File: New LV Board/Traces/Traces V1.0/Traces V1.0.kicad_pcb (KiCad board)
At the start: 6 copper layers, 105.7 x 51.8 mm, 15 parts, among them J1 B15B-PH-K-S, J2 B15B-PH-K-S, J3 B15B-PH-K-S, J4 Conn_01x12, J6 Conn_01x12, J7 Conn_01x12

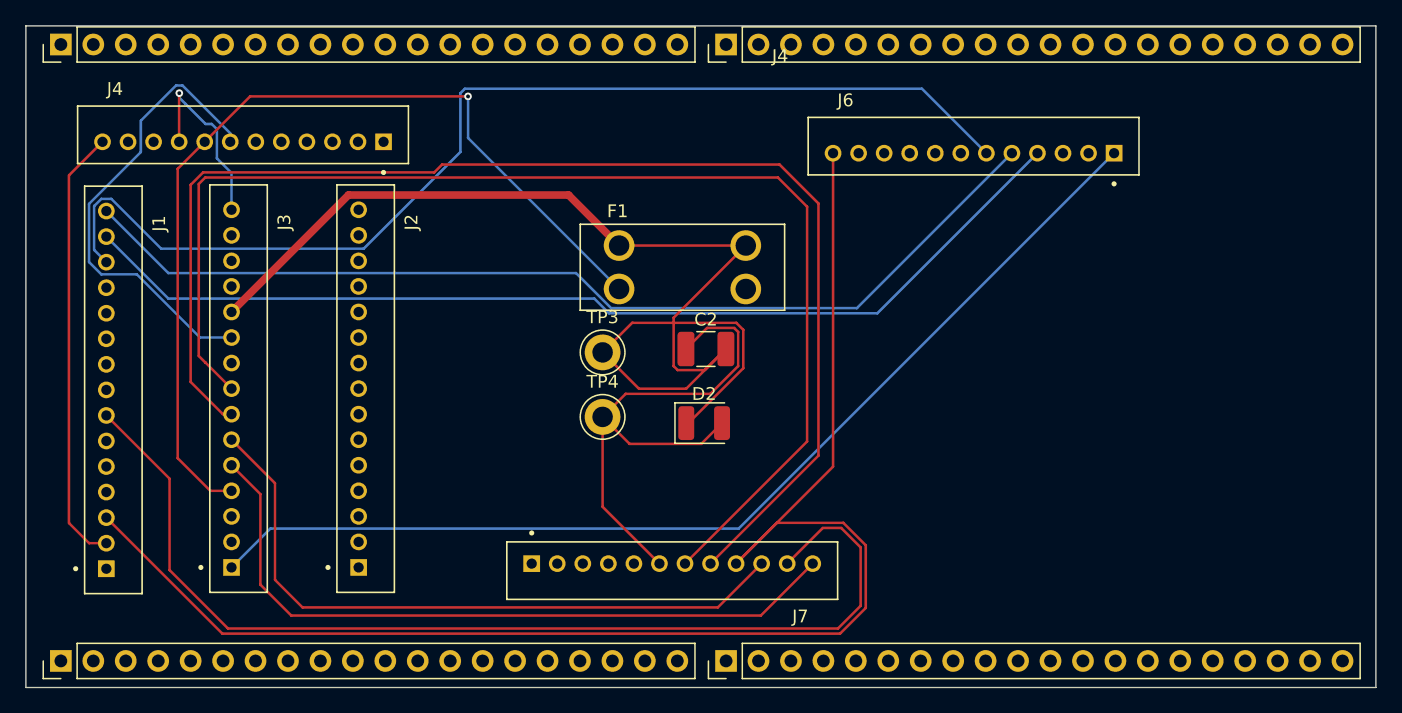
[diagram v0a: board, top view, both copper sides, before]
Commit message: traces probably
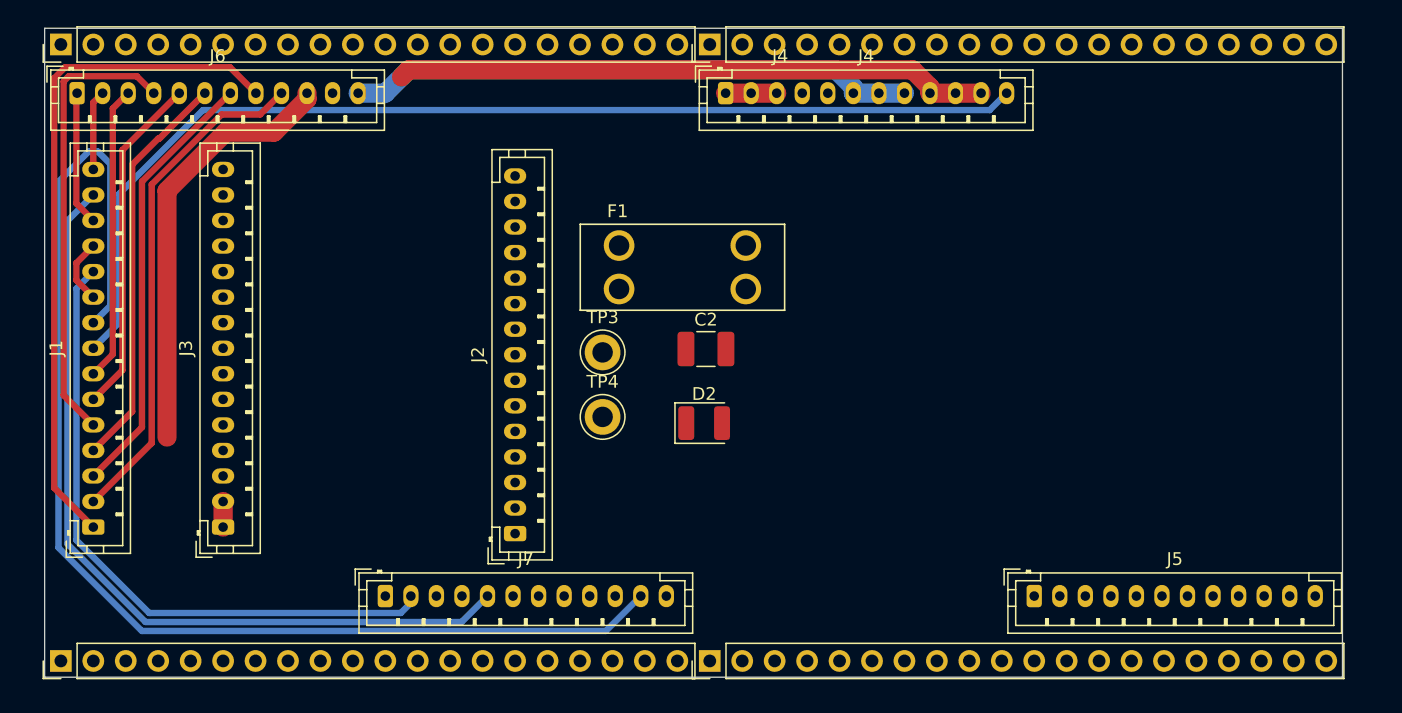
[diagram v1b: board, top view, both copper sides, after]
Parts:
- added J5: B12B-PH-K-S, Connector_JST:JST_PH_B12B-PH-K_1x12_P2.00mm_Vertical, F.Cu at (116.8, 104.1)
- J1, J2, J3: footprint motorsports:JST_B15B-PH-K-S -> Connector_JST:JST_PH_B15B-PH-K_1x15_P2.00mm_Vertical
- J4, J6, J7: value Conn_01x12 -> B12B-PH-K-S; footprint motorsports:JST_B12B-PH-K-S -> Connector_JST:JST_PH_B12B-PH-K_1x12_P2.00mm_Vertical
- moved J6 70.3 mm to (41.9, 64.8)
- moved J4 37.9 mm to (92.7, 64.8)
- moved J7 22.5 mm to (66.0, 104.1), turned to 0 degrees
- moved J2 16.3 mm to (76.2, 99.2), turned to 90 degrees
- moved J3 10.9 mm to (53.3, 98.7), turned to 90 degrees
- moved J1 10.9 mm to (43.2, 98.7), turned to 90 degrees
- moved REF** 1.28 mm to (91.4, 61.0)
- moved REF** 1.28 mm to (91.4, 109.2)
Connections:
- F1 pad 3: Net-(J4-Pin_8) -> Net-(J4-Pin_5)
- F1 pad 4: Net-(J4-Pin_8) -> Net-(J4-Pin_5)
- J1 pad 1: Net-(J6-Pin_11) -> Net-(J6-Pin_8)
- J1 pad 10: Net-(J6-Pin_8) -> Net-(J1-Pad10)
- J1 pad 11: Net-(J6-Pin_9) -> Net-(J7-Pin_2)
- J1 pad 12: Net-(J6-Pin_7) -> Net-(J1-Pad10)
- J1 pad 13: Net-(J6-Pin_6) -> Net-(J6-Pin_1)
- J1 pad 14: Net-(J6-Pin_4) -> Net-(J4-Pin_1)
- J1 pad 15: Net-(J6-Pin_5) -> Net-(J6-Pin_2)
- J1 pad 2: Net-(J4-Pin_10) -> Net-(J6-Pin_9)
- J1 pad 3: Net-(J6-Pin_12) -> Net-(J6-Pin_7)
- J1 pad 4: unconnected-(J1-Pad4) -> Net-(J6-Pin_6)
- J1 pad 5: unconnected-(J1-Pad5) -> Net-(J6-Pin_4)
- J1 pad 6: unconnected-(J1-Pad6) -> Net-(J6-Pin_5)
- J1 pad 7: Net-(J7-Pin_11) -> Net-(J6-Pin_3)
- J1 pad 8: Net-(J4-Pin_1) -> Net-(J4-Pin_12)
- J1 pad 9: Net-(J6-Pin_10) -> Net-(J7-Pin_11)
- J2 pad 1: unconnected-(J2-Pad1) -> Net-(J7-Pin_3)
- J2 pad 2: unconnected-(J2-Pad2) -> Net-(J7-Pin_4)
- J2 pad 5: unconnected-(J2-Pad5) -> Net-(J5-Pin_9)
- J2 pad 6: unconnected-(J2-Pad6) -> Net-(J5-Pin_8)
- J2 pad 7: unconnected-(J2-Pad7) -> Net-(J5-Pin_7)
- J2 pad 8: unconnected-(J2-Pad8) -> Net-(J5-Pin_6)
- J3 pad 1: Net-(J4-Pin_5) -> Net-(D2-A)
- J3 pad 10: Net-(J4-Pin_5) -> Net-(J7-Pin_10)
- J3 pad 11: Net-(D2-K) -> Net-(J7-Pin_12)
- J3 pad 12: Net-(D2-K) -> Net-(J4-Pin_5)
- J3 pad 13: Net-(D2-K) -> unconnected-(J3-Pad13)
- J3 pad 14: Net-(D2-A) -> unconnected-(J3-Pad14)
- J3 pad 15: Net-(D2-A) -> Net-(J4-Pin_6)
- J3 pad 2: unconnected-(J3-Pad2) -> Net-(D2-A)
- J3 pad 3: unconnected-(J3-Pad3) -> Net-(D2-K)
- J3 pad 4: Net-(J4-Pin_8) -> Net-(D2-K)
- J3 pad 5: Net-(J7-Pin_12) -> Net-(D2-K)
- J3 pad 6: Net-(J7-Pin_10) -> Net-(J4-Pin_6)
- J3 pad 7: Net-(J7-Pin_8) -> Net-(J4-Pin_6)
- J3 pad 9: Net-(J4-Pin_5) -> Net-(J7-Pin_8)
- J4 pad 10: Net-(J4-Pin_10) -> Net-(D2-K)
- J4 pad 11: Net-(J4-Pin_10) -> Net-(D2-K)
- J4 pad 12: Net-(J4-Pin_10) -> Net-(J4-Pin_12)
- J4 pad 2: Net-(D2-K) -> Net-(J4-Pin_1)
- J4 pad 3: Net-(D2-K) -> Net-(J4-Pin_1)
- J4 pad 4: Net-(D2-K) -> Net-(D2-A)
- J4 pad 6: Net-(J4-Pin_5) -> Net-(J4-Pin_6)
- J4 pad 7: Net-(J4-Pin_5) -> Net-(J4-Pin_6)
- J4 pad 8: Net-(J4-Pin_8) -> Net-(J4-Pin_6)
- J4 pad 9: Net-(D2-A) -> Net-(D2-K)
- J6 pad 1: Net-(J4-Pin_5) -> Net-(J6-Pin_1)
- J6 pad 10: Net-(J6-Pin_10) -> Net-(D2-A)
- J6 pad 11: Net-(J6-Pin_11) -> Net-(J4-Pin_5)
- J6 pad 12: Net-(J6-Pin_12) -> Net-(J4-Pin_6)
- J6 pad 2: Net-(J4-Pin_8) -> Net-(J6-Pin_2)
- J6 pad 3: Net-(D2-A) -> Net-(J6-Pin_3)
- J7 pad 2: unconnected-(J7-Pin_2-Pad2) -> Net-(J7-Pin_2)
- J7 pad 3: unconnected-(J7-Pin_3-Pad3) -> Net-(J7-Pin_3)
- J7 pad 4: unconnected-(J7-Pin_4-Pad4) -> Net-(J7-Pin_4)
- J7 pad 5: Net-(J4-Pin_10) -> Net-(J4-Pin_1)
- J7 pad 9: Net-(J6-Pin_12) -> Net-(J6-Pin_1)
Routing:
- net Net-(J4-Pin_8): track 200.2 -> 0.00 mm, vias 1 -> 0
- net Net-(J4-Pin_5): track 159.0 -> 0.00 mm
- net Net-(D2-A): track 168.9 -> 35.7 mm, vias 1 -> 0
- net Net-(J6-Pin_12): track 116.4 -> 0.00 mm
- net Net-(J7-Pin_8): track 102.4 -> 0.00 mm
- net Net-(J7-Pin_7): track 97.8 -> 0.00 mm
- net Net-(D2-K): track 141.7 -> 46.6 mm
- net Net-(J6-Pin_11): track 91.9 -> 0.00 mm
- net Net-(J4-Pin_12): track 0.00 -> 85.7 mm
- net Net-(J6-Pin_10): track 84.0 -> 0.00 mm
- net Net-(J4-Pin_10): track 80.7 -> 0.00 mm
- net Net-(J7-Pin_12): track 56.2 -> 0.00 mm
- net Net-(J6-Pin_6): track 86.5 -> 31.6 mm
- net Net-(J7-Pin_10): track 52.8 -> 0.00 mm
- net Net-(J6-Pin_5): track 79.1 -> 26.8 mm, vias 0 -> 1
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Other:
- board size 105.7 x 51.8 mm -> 101.6 x 50.8 mm
- copper layers 6 -> 4
